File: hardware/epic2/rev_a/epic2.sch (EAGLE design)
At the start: 35 parts, among them J1 EPIC2-HEADER2, U2 FM25LBTDFN-8, U3 CC2538, U5 RV-3049-C3, X1 EPSON-FA-128, X3 ABS05-32.768KHZ-T

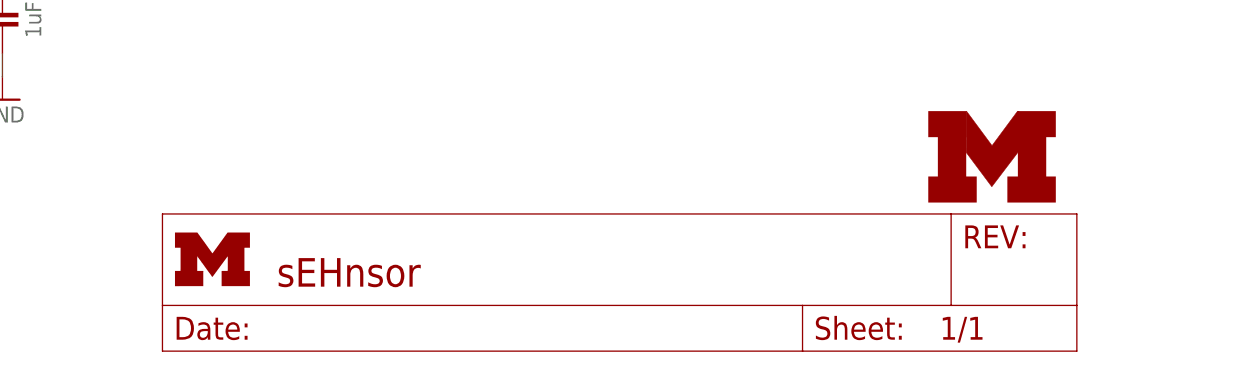
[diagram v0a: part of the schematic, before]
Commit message: epic2: cleaned up a couple things
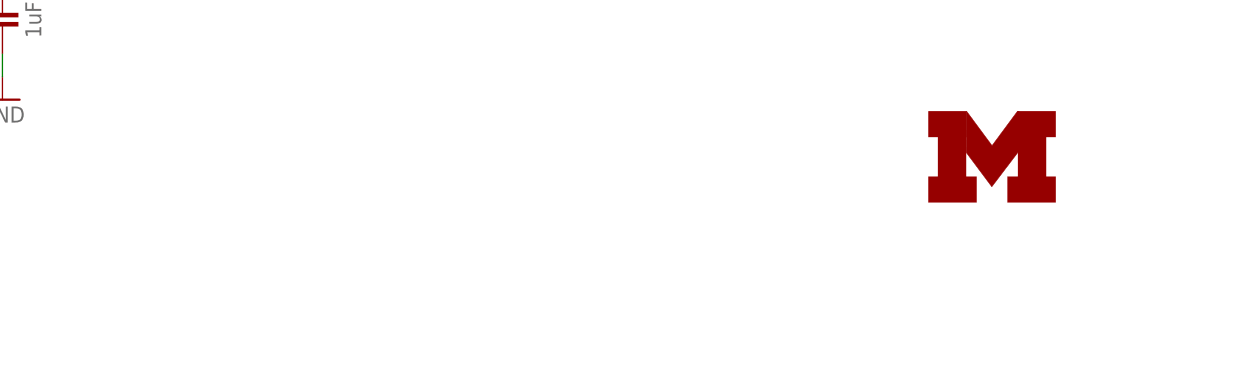
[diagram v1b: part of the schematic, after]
